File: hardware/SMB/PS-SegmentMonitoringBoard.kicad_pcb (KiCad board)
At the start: 4 copper layers, 83.9 x 80.3 mm, 110 parts, among them IC1 BQ79616PAPR, J1 voltTapsConn, J2 highSideConn, J3 lowSideConn, J4 thermsConn, Q1 ZXTN4004KTC

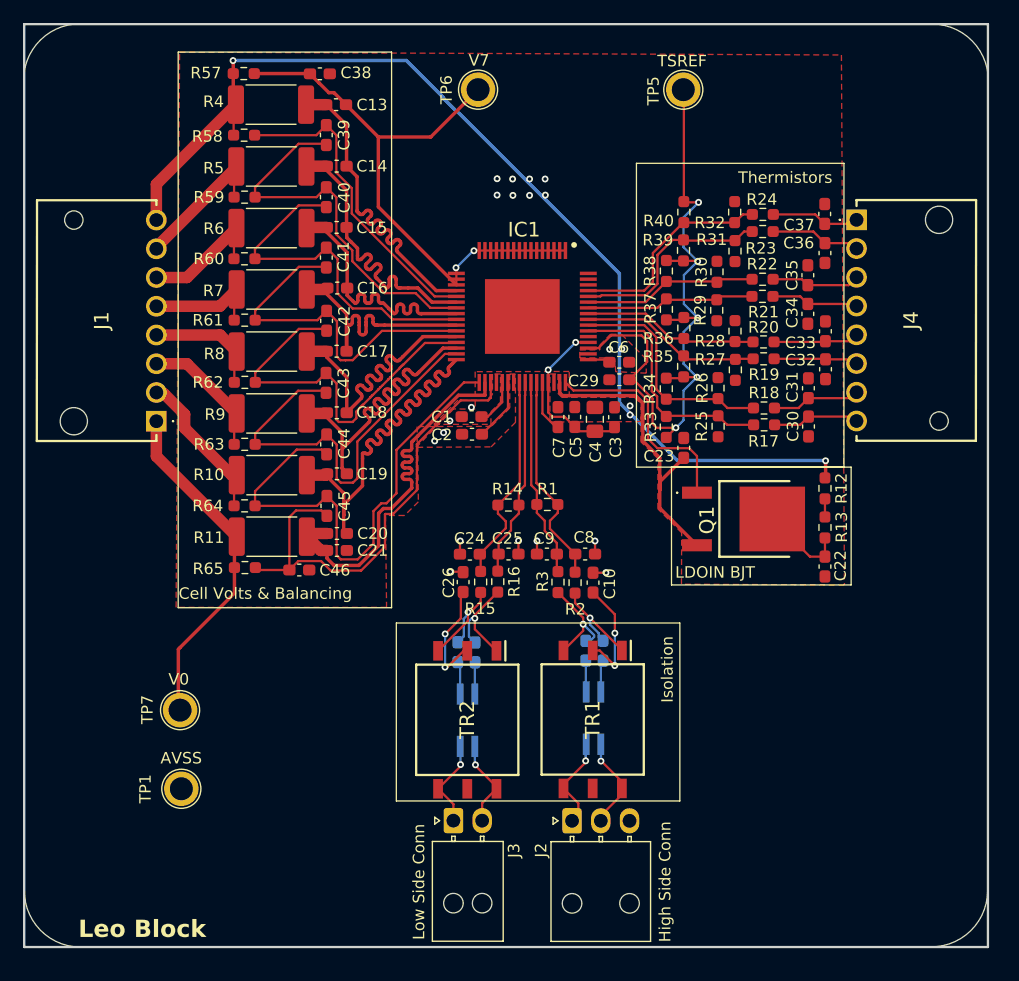
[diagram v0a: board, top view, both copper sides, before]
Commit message: layout v3, everything done
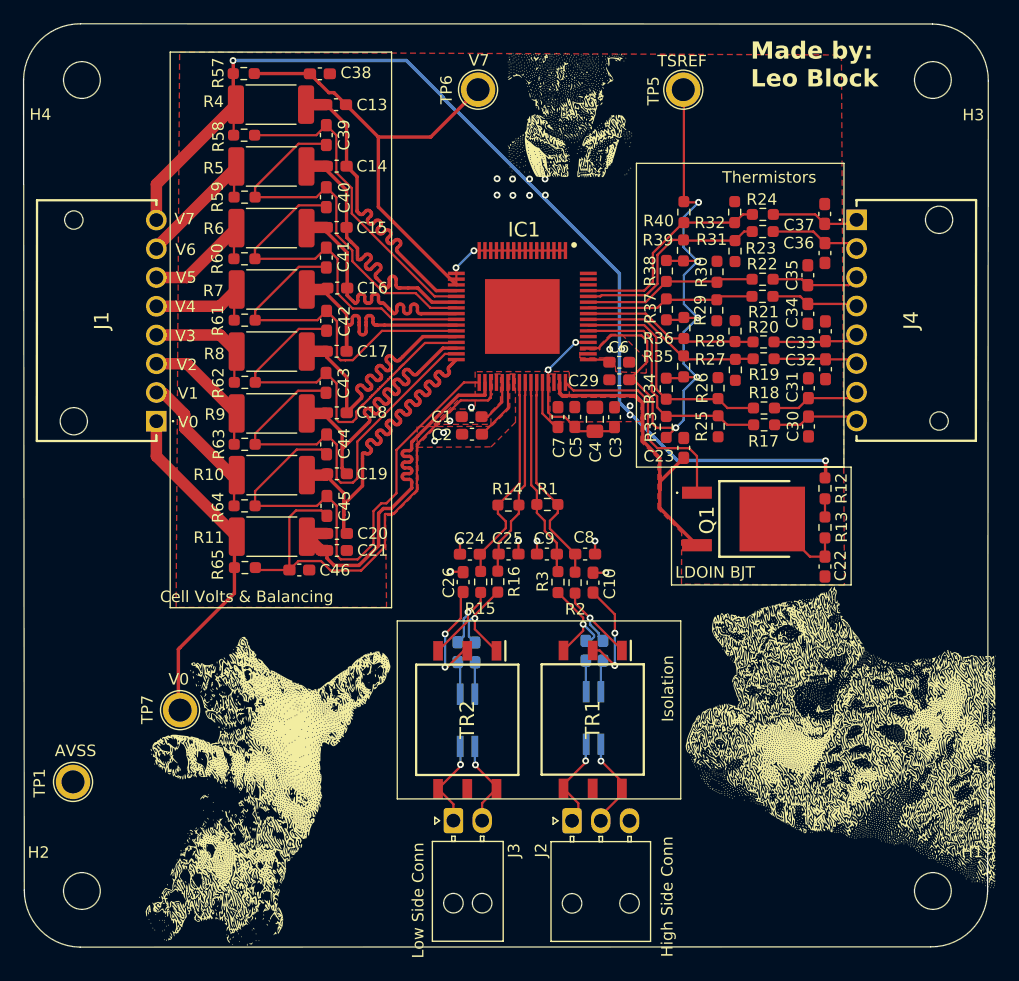
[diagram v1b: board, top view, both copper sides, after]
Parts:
- added G***: LOGO, LOGO, F.Cu at (145.1, 125.0)
- added G***: LOGO, LOGO, F.Cu at (121.6, 71.0)
- added G***: LOGO, LOGO, F.Cu at (95.4, 129.9)
- added G***: LOGO, LOGO, B.Cu at (144.9, 123.4)
- added G***: LOGO, LOGO, B.Cu at (124.6, 84.1)
- added G***: LOGO, LOGO, B.Cu at (89.3, 122.8)
- added H1: MountingHole, MountingHole:MountingHole_3.2mm_M3, F.Cu at (153.2, 138.5)
- added H2: MountingHole, MountingHole:MountingHole_3.2mm_M3, F.Cu at (79.2, 138.5)
- added H3: MountingHole, MountingHole:MountingHole_3.2mm_M3, F.Cu at (153.2, 67.9)
- added H4: MountingHole, MountingHole:MountingHole_3.2mm_M3, F.Cu at (79.2, 67.9)
- moved TP1 9.44 mm to (78.4, 129.0), turned to 90 degrees
- moved LOGO1 5.03 mm to (141.2, 141.0)
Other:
- outline, holes or cut-outs redrawn
- board text added: "Made by: Leo Block"
- board text added: "V1"
- board text added: "V2"
- board text added: "V3"
- board text added: "V4"
- board text added: "V5"
- board text added: "V6"
- board text removed: "Leo Block"
